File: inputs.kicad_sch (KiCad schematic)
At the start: 62 parts, among them J4 TPS43, SW1 KEY_A, SW10 D2F-01F, SW11 D2F-01F, SW12 D2F-01F, SW13 RKB2SJM250SMTR LFS, SW14 RKB2SJM250SMTR LFS, SW15 RKB2SJM250SMTR LFS, SW2 KEY_B, SW3 KEY_C, SW4 KEY_D, SW5 KEY_E, SW6 KEY_F, SW7 D2F-01F, SW8 D2F-01F, SW9 D2F-01F

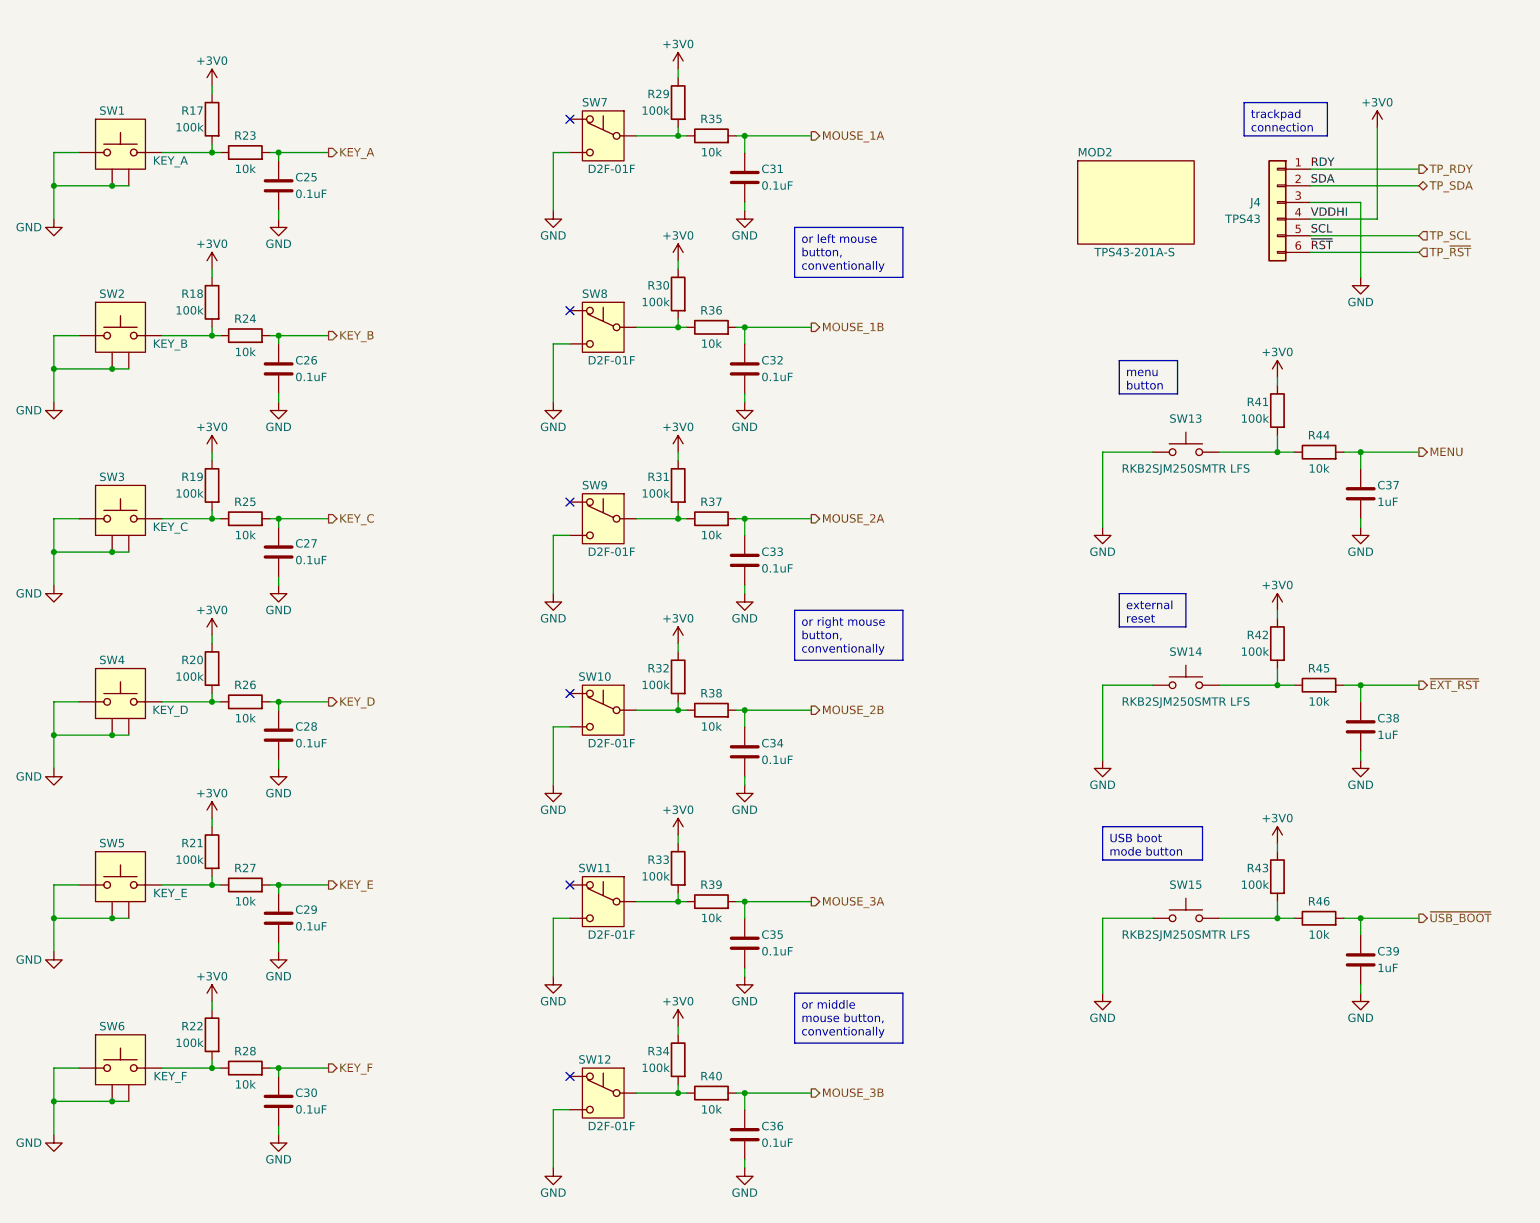
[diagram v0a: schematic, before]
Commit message: schematic cleanup
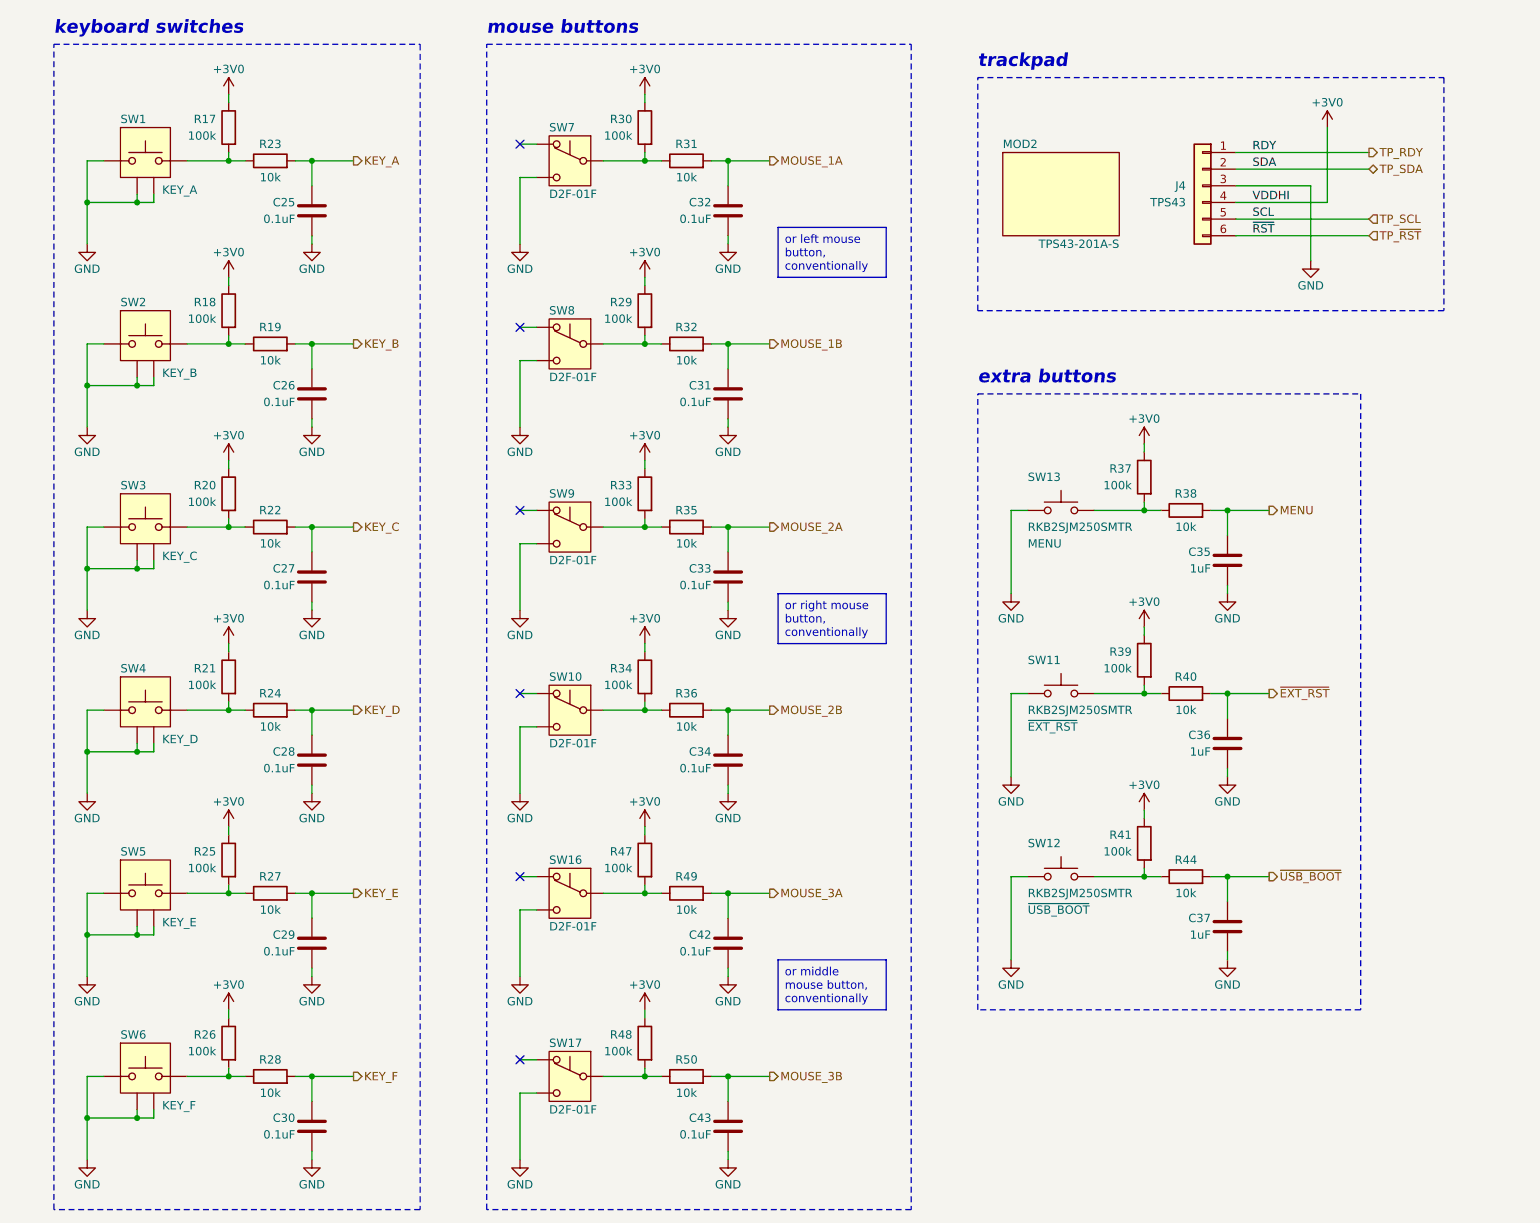
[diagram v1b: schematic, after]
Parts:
- removed C38, C39: 1uF, Capacitor_SMD:C_0805_2012Metric, symbol Device:C
- removed R42, R43: 100k, Resistor_SMD:R_0805_2012Metric, symbol Device:R
- removed R45, R46: 10k, Resistor_SMD:R_0805_2012Metric, symbol Device:R
- removed SW11, SW12: D2F-01F, footprints:D2F01F, symbol user:D2F-01F
- removed SW14, SW15: RKB2SJM250SMTR LFS, footprints:RKB2SJM250SMTRLFS, symbol Switch:SW_Push
- added C42, C43: 0.1uF, Capacitor_SMD:C_0805_2012Metric, symbol Device:C
- added R47, R48: 100k, Resistor_SMD:R_0805_2012Metric, symbol Device:R
- added R49, R50: 10k, Resistor_SMD:R_0805_2012Metric, symbol Device:R
- added SW11, SW12: RKB2SJM250SMTR, footprints:RKB2SJM250SMTRLFS, symbol Switch:SW_Push
- added SW16, SW17: D2F-01F, footprints:D2F01F, symbol user:D2F-01F
- C35, C36: value 0.1uF -> 1uF
- R19, R22, R31, R32: value 100k -> 10k
- R25, R26, R37, R39: value 10k -> 100k
- SW13: value RKB2SJM250SMTR LFS -> RKB2SJM250SMTR; Input (none) -> MENU
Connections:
- net +3V0: now also R25.1, R26.1, R37.1, R39.1, R47.1, R48.1; no longer R19.1, R22.1, R31.1, R32.1
- net GND: now also C42.2, C43.2, SW11.1, SW12.1, SW16.2 (NO), SW17.2 (NO)
- net KEY_B: now also R19.2; no longer R24.2
- net KEY_C: now also R22.2; no longer R25.2
- net KEY_D: now also R24.2; no longer R26.2
- net MENU: now also C35.1, R38.2; no longer C37.1, R44.2
- net MOUSE_1A: now also C32.1, R31.2; no longer C31.1, R35.2
- net MOUSE_1B: now also C31.1, R32.2; no longer C32.1, R36.2
- net MOUSE_2A: now also R35.2; no longer R37.2
- net MOUSE_2B: now also R36.2; no longer R38.2
- net MOUSE_3A: now also C42.1, R49.2; no longer C35.1, R39.2
- net MOUSE_3B: now also C43.1, R50.2; no longer C36.1, R40.2
- net ~{EXT_RST}: now also C36.1, R40.2
- net ~{USB_BOOT}: now also C37.1, R44.2
- net at R18.2, SW2.2: now also R19.1; no longer R24.1
- net at R28.1, SW6.2: now also R26.2; no longer R22.2
- net at R34.2: now also R36.1, SW10.1 (COM); no longer R40.1
- net at R27.1, SW5.2: now also R25.2; no longer R21.2
- net at R33.2: now also R35.1, SW9.1 (COM); no longer R39.1
- net at R41.2, R44.1: now also SW12.2; no longer SW13.2
- new net: R48.2, R50.1, SW17.1 (COM)
- new net: R30.2, R31.1, SW7.1 (COM)
- new net: R37.2, R38.1, SW13.2
- new net: R20.2, R22.1, SW3.2
- new net: R47.2, R49.1, SW16.1 (COM)
- new net: R21.2, R24.1, SW4.2
- new net: R39.2, R40.1, SW11.2
- new net: R29.2, R32.1, SW8.1 (COM)
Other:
- note added: "extra buttons"
- note added: "keyboard switches"
- note added: "mouse buttons"
- note added: "trackpad"
- moved on the sheet: C25, J4, MOD2, R17, R23, SW1, SW13, SW7
